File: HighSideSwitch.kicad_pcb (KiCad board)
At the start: 2 copper layers, 22 x 15.1 mm, 24 parts, among them J1 Conn_02x02_Odd_Even, Q1 CSD18540Q5B, Q2 CSD18540Q5B, Q3 8050, U1 LM5060, U2 LM5050-1

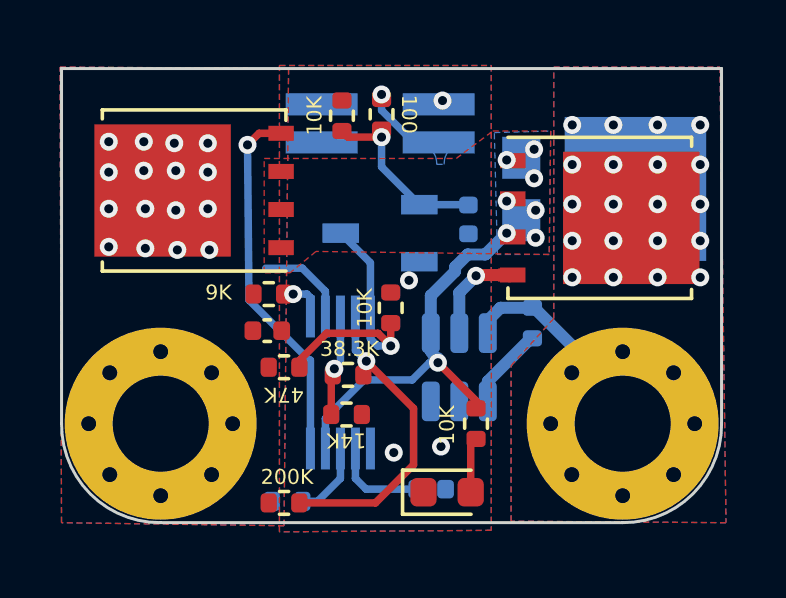
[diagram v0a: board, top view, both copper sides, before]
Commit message: reset
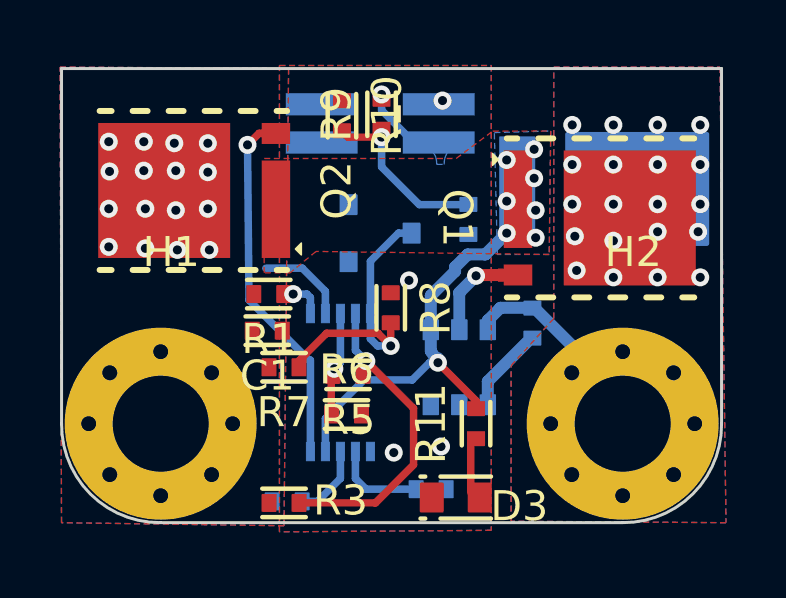
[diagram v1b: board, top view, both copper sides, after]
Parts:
- removed D2: LED, LED_SMD:LED_0603_1608Metric
- added D3: LED, GENERAL_2-PIN_PLASTIC_SMD:LED0603(1608M), F.Cu at (189.3, 93.9)
- C1, C3, C4: footprint Capacitor_SMD:C_0402_1005Metric -> GENERAL_RCL_SMD:C0402(1005M)
- D1: value VS-6ESU06 -> Diode; footprint Package_TO_SOT_SMD:TO-277A -> POWER_DIODE_SMD:TO-277A
- H1, H2: value MountingHole_Pad -> MountingHole; footprint MountingHole:MountingHole_3.2mm_M3_Pad_Via -> MOUNTINGHOLE:MountingHole
- J1: value Conn_02x02_Odd_Even -> Conn_02x02; footprint Connector_PinHeader_1.27mm:PinHeader_2x02_P1.27mm_Vertical_SMD -> CONNECTOR:Conn-02x02
- Q1, Q2: value CSD18540Q5B -> CSD18540; footprint Package_TO_SOT_SMD:TDSON-8-1 -> POWER_TRANSISTOR_SMD:SON-6050-FET
- Q3: footprint Package_TO_SOT_SMD:TSOT-23 -> GENERAL_SMALL-SEMI_SMD:SOT-23
- R1, R10, R11, R2, R3, R4, R5, R6, R7, R8, R9: footprint Resistor_SMD:R_0402_1005Metric -> GENERAL_RCL_SMD:R0402(1005M)
- U1: footprint Package_SO:MSOP-10_3x3mm_P0.5mm -> GENERAL_MIDDLE-SEMI_SMD:MSOP-3030_10
- U2: footprint Package_TO_SOT_SMD:TSOT-23-6 -> GENERAL_SMALL-SEMI_SMD:SOT-23-6
- turned D1 to 180 degrees
- turned Q1 to -90 degrees
- turned Q2 to 90 degrees
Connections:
- C3 pad 1: Net-(C3-Pad1) -> GND
- C3 pad 2: GND -> Net-(C3-Pad2)
- C4 pad 1: Net-(C4-Pad1) -> GND
- C4 pad 2: GND -> Net-(C4-Pad2)
- H1 pad 1: /NMOS_IN -> (no net)
- H2 pad 1: /NMOS_OUT -> (no net)
- Q3 pad 1: Net-(C4-Pad1) -> Net-(C4-Pad2)
- R10 pad 1: Net-(C4-Pad1) -> GND
- R10 pad 2: GND -> Net-(C4-Pad2)
- R11 pad 1: Net-(D1-Pad1) -> Net-(D3-PadA)
- R11 pad 2: Net-(D2-Pad2) -> Net-(Q2-Pad2)
- R3 pad 1: /NMOS_IN -> Net-(R3-Pad1)
- R3 pad 2: Net-(R3-Pad2) -> /NMOS_IN
- R5 pad 1: Net-(R5-Pad1) -> Net-(R3-Pad1)
- R5 pad 2: Net-(R3-Pad2) -> Net-(R5-Pad2)
- R6 pad 2: Net-(R5-Pad1) -> Net-(R5-Pad2)
- R7 pad 1: /NMOS_IN -> /EN
- R7 pad 2: /EN -> /NMOS_IN
- R9 pad 2: Net-(C4-Pad1) -> Net-(C4-Pad2)
- U1 pad 10: Net-(Q2-Pad4) -> Net-(Q2-Pad1)
- U1 pad 3: Net-(R5-Pad1) -> Net-(R5-Pad2)
- U1 pad 4: Net-(R3-Pad2) -> Net-(R3-Pad1)
- U1 pad 7: Net-(C3-Pad1) -> Net-(C3-Pad2)
- U1 pad 9: Net-(D1-Pad1) -> Net-(Q2-Pad2)
- U2 pad 4: Net-(D1-Pad1) -> Net-(Q2-Pad2)
- U2 pad 5: Net-(Q1-Pad4) -> Net-(Q1-Pad1)
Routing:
- net Net-(D1-Pad1): track 13.5 -> 0.00 mm, vias 8 -> 0
- net /NMOS_OUT: track 7.23 -> 20.7 mm, vias 20 -> 28
- net Net-(R5-Pad2): track 0.00 -> 13.2 mm, vias 0 -> 2
- net GND: track 0.00 -> 12.4 mm, vias 4 -> 6
- net Net-(Q2-Pad4): track 12.3 -> 0.00 mm, vias 1 -> 0
- net Net-(Q2-Pad1): track 0.00 -> 12.3 mm, vias 0 -> 1
- net Net-(R3-Pad2): track 10.1 -> 0.00 mm, vias 1 -> 0
- net Net-(C4-Pad1): track 5.82 -> 0.00 mm, vias 1 -> 0
- net Net-(Q1-Pad4): track 3.38 -> 0.00 mm, vias 1 -> 0
- net Net-(C3-Pad1): track 3.19 -> 0.00 mm
- net Net-(R5-Pad1): track 3.17 -> 0.00 mm, vias 1 -> 0
- net Net-(Q2-Pad2): track 0.00 -> 1.85 mm
- net Net-(D2-Pad2): track 1.85 -> 0.00 mm
- added copper zone on B.Cu, net Net-(Q2-Pad2)
- added copper zone on F.Cu, net Net-(Q2-Pad2)
- removed copper zone on B.Cu, net Net-(D1-Pad1)
- removed copper zone on F.Cu, net Net-(D1-Pad1)

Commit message: final
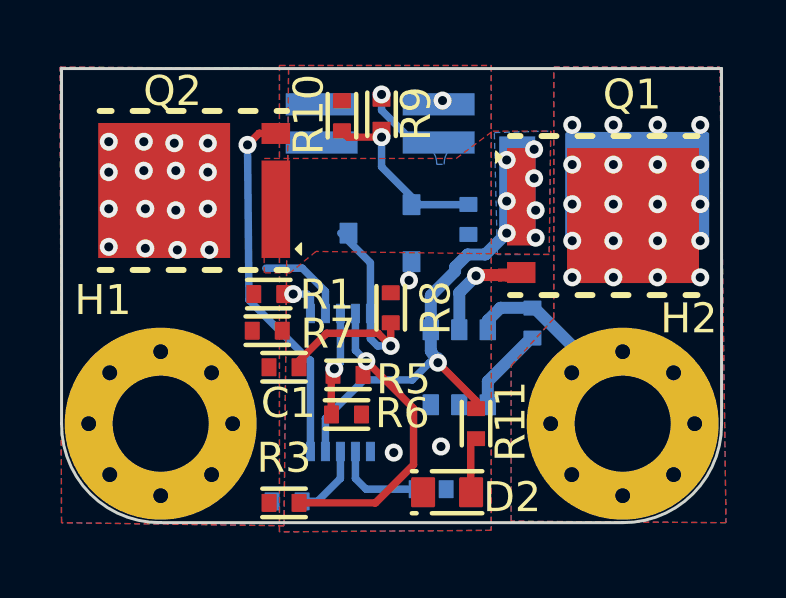
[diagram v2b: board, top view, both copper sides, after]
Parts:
- removed D3: LED, GENERAL_2-PIN_PLASTIC_SMD:LED0603(1608M)
- added D2: Diode_LED, GENERAL_2-PIN_PLASTIC_SMD:LED0603(1608M), F.Cu at (189.0, 93.7)
- Q1, Q2: value CSD18540 -> CSD18540Q5B
- moved Q1 0.13 mm to (194.2, 84.5)
- turned C3 to 180 degrees
- turned C4 to 90 degrees
- turned Q3 to 0 degrees
- turned R10 to -90 degrees
- turned R11 to 90 degrees
- turned R3 to 180 degrees
- turned R5 to 180 degrees
- turned R7 to 180 degrees
- turned U2 to -90 degrees
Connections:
- H1 pad 1: (no net) -> /NMOS_IN
- H2 pad 1: (no net) -> /NMOS_OUT
- Q1 pad D: (no net) -> /NMOS_OUT
- Q1 pad G: (no net) -> Net-(Q1-PadG)
- Q1 pad S: (no net) -> Net-(D1-PadA)
- Q2 pad G: (no net) -> Net-(Q2-PadG)
- Q2 pad S: (no net) -> Net-(D1-PadA)
- R11 pad 2: Net-(Q2-Pad2) -> Net-(D1-PadA)
- U1 pad 10: Net-(Q2-Pad1) -> Net-(Q2-PadG)
- U1 pad 9: Net-(Q2-Pad2) -> Net-(D1-PadA)
- U2 pad 4: Net-(Q2-Pad2) -> Net-(D1-PadA)
- U2 pad 5: Net-(Q1-Pad1) -> Net-(Q1-PadG)
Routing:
- net Net-(D1-PadA): track 0.00 -> 13.5 mm, vias 0 -> 8
- net /NMOS_OUT: track 20.7 -> 7.23 mm, vias 28 -> 20
- net GND: track 12.4 -> 0.00 mm, vias 6 -> 4
- net Net-(Q2-PadG): track 0.00 -> 12.3 mm, vias 0 -> 1
- net Net-(Q2-Pad1): track 12.3 -> 0.00 mm, vias 1 -> 0
- net Net-(R5-Pad2): track 13.2 -> 3.17 mm, vias 2 -> 1
- net Net-(R3-Pad1): track 0.00 -> 10.1 mm, vias 0 -> 1
- net Net-(C4-Pad2): track 0.00 -> 5.82 mm, vias 0 -> 1
- net Net-(Q1-PadG): track 0.00 -> 3.38 mm, vias 0 -> 1
- net Net-(C3-Pad2): track 0.00 -> 3.19 mm
- net Net-(Q2-Pad2): track 1.85 -> 0.00 mm
- net Net-(D2-Pad2): track 0.00 -> 1.85 mm
- added copper zone on B.Cu, net Net-(D1-PadA)
- added copper zone on F.Cu, net Net-(D1-PadA)
- removed copper zone on B.Cu, net Net-(Q2-Pad2)
- removed copper zone on F.Cu, net Net-(Q2-Pad2)
